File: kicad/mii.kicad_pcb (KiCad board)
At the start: 2 copper layers, 25.7 x 42.9 mm, 8 parts, among them IC1 RFM69, J1 Conn_Coaxial, J2 Conn_01x05, J3 Conn_01x03, J4 Conn_01x03, J5 Conn_01x03, J6 Conn_01x05, U1 WeMos_mini

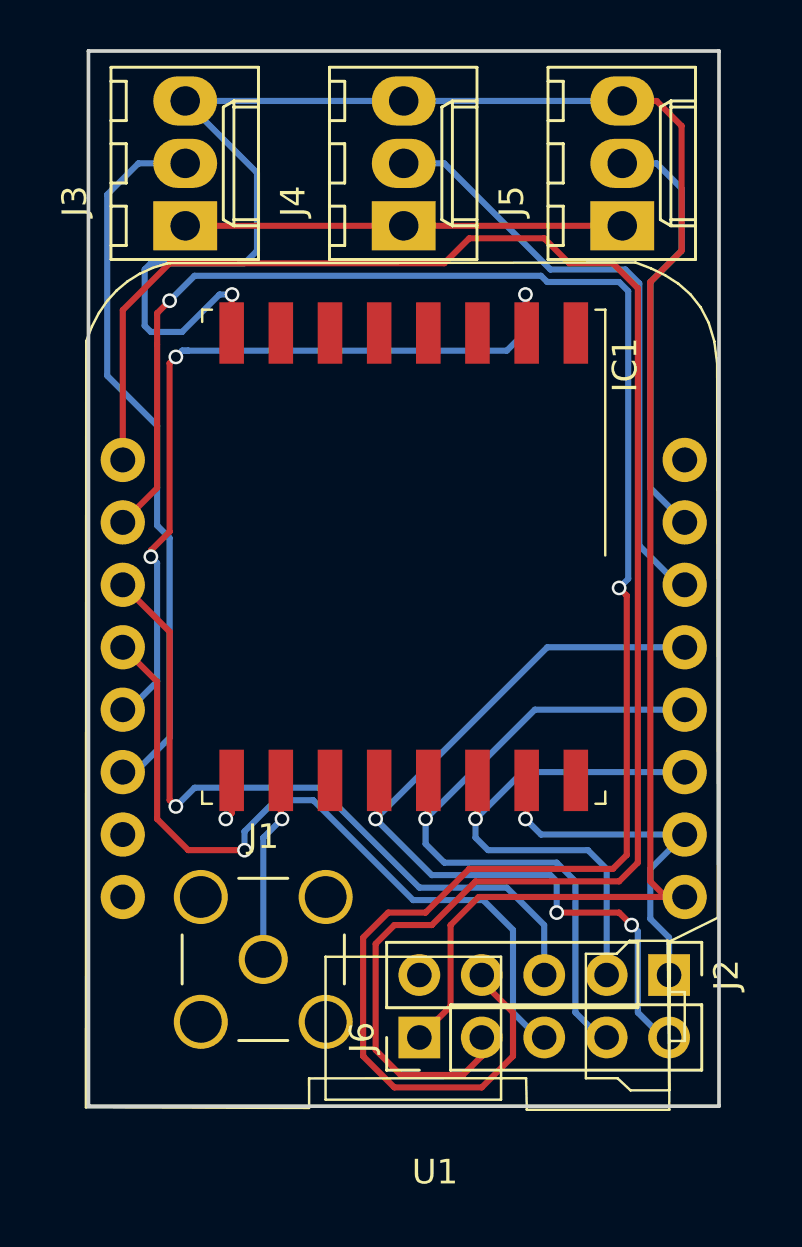
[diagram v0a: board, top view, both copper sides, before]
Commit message: Fix boundaries
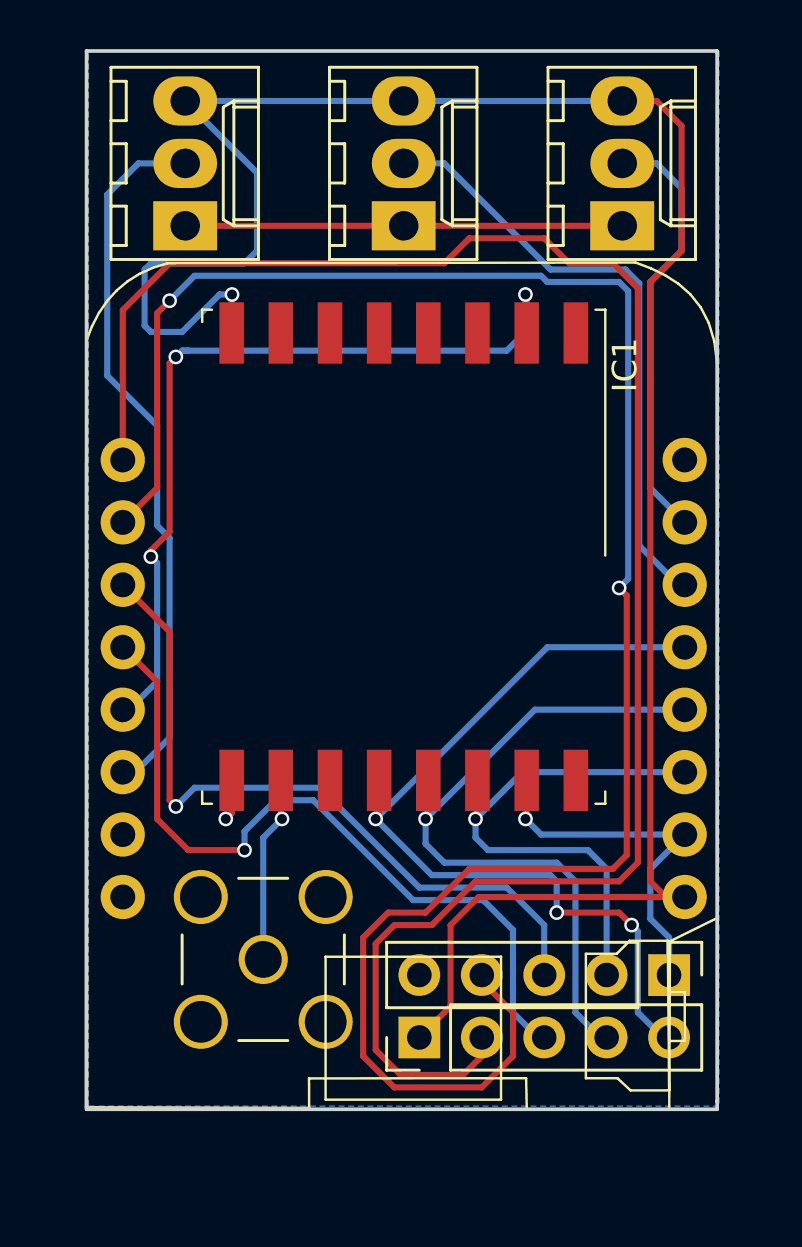
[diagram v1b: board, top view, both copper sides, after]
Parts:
- J1: value Conn_Coaxial -> Coaxial
- J2: value Conn_01x05 -> 3.3 TX SCL MISO SCK
- J3: value Conn_01x03 -> GND D4 3.3
- J4: value Conn_01x03 -> GND D0 3.3
- J5: value Conn_01x03 -> GND A0 3.3
- J6: value Conn_01x05 -> GND RX SDA MOSI NSS
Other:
- board size 25.7 x 42.9 mm -> 25.7 x 43.1 mm
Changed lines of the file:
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@@
     (area 106.92 82.88238 135.75 129.74)
     (thickness 1.6)
-    (drawings 4)
+    (drawings 6)
     (tracks 195)
     (zones 0)
@@
     (descr "Through hole straight pin header, 1x05, 2.54mm pitch, single row")
     (tags "Through hole pin header THT 1x05 2.54mm single row")
-    (fp_text reference J6 (at 0 -2.33 90) (layer F.SilkS)
-      (effects (font (size 1 1) (thickness 0.15)))
-    )
-    (fp_text value Conn_01x05 (at 0 12.49 90) (layer F.Fab)
-      (effects (font (size 1 1) (thickness 0.15)))
+    (fp_text reference J6 (at 0 -2.33 90) (layer F.SilkS) hide
+      (effects (font (size 1 1) (thickness 0.15)))
+    )
+    (fp_text value "GND RX SDA MOSI NSS" (at 4.318 5.08 180) (layer F.Fab)
+      (effects (font (size 0.7 0.7) (thickness 0.15)))
     )
     (fp_line (start -0.635 -1.27) (end 1.27 -1.27) (layer F.Fab) (width 0.1))
@@
   (module wemos_d1_mini:D1_mini_board (layer F.Cu)
     (at 121.285 109.855)
-    (fp_text reference U1 (at 1.27 18.81) (layer F.SilkS)
-      (effects (font (size 1 1) (thickness 0.15)))
-    )
-    (fp_text value WeMos_mini (at 1.27 -19.05) (layer F.Fab)
+    (fp_text reference U1 (at 1.27 18.81) (layer F.SilkS) hide
+      (effects (font (size 1 1) (thickness 0.15)))
+    )
+    (fp_text value WeMos_mini (at 1.27 -19.05) (layer F.Fab) hide
       (effects (font (size 1 1) (thickness 0.15)))
     )
@@
     (descr "Connector Headers with Friction Lock, 22-27-2031, http://www.molex.com/pdm_docs/sd/022272021_sd.pdf")
     (tags "connector molex kk_6410 22-27-2031")
-    (fp_text reference J3 (at 1 -4.5 90) (layer F.SilkS)
-      (effects (font (size 1 1) (thickness 0.15)))
-    )
-    (fp_text value Conn_01x03 (at 2.54 4.5 90) (layer F.Fab)
-      (effects (font (size 1 1) (thickness 0.15)))
+    (fp_text reference J3 (at 1 -4.5 90) (layer F.SilkS) hide
+      (effects (font (size 1 1) (thickness 0.15)))
+    )
+    (fp_text value "GND  D4 3.3" (at 2.286 -1.905 90) (layer F.Fab)
+      (effects (font (size 0.7 0.7) (thickness 0.15)))
     )
     (fp_line (start -1.47 -3.12) (end -1.47 3.08) (layer F.Fab) (width 0.12))
@@
     (fp_line (start 7 -3.55) (end 7 3.5) (layer F.CrtYd) (width 0.05))
     (fp_line (start 7 3.5) (end -1.9 3.5) (layer F.CrtYd) (width 0.05))
-    (fp_text user %R (at 2.54 0 90) (layer F.Fab)
+    (fp_text user %R (at 5.588 2.413 90) (layer F.Fab)
       (effects (font (size 1 1) (thickness 0.15)))
     )
@@
     (descr "SMA pcb through hole jack")
     (tags "SMA THT Jack Straight")
-    (fp_text reference J1 (at 0 -5) (layer F.SilkS)
-      (effects (font (size 1 1) (thickness 0.15)))
-    )
-    (fp_text value Conn_Coaxial (at 0 5) (layer F.Fab)
+    (fp_text reference J1 (at 0 -5) (layer F.SilkS) hide
+      (effects (font (size 1 1) (thickness 0.15)))
+    )
+    (fp_text value Coaxial (at 0 5) (layer F.Fab)
       (effects (font (size 1 1) (thickness 0.15)))
     )
@@
     (fp_line (start -1 -3.3) (end 1 -3.3) (layer F.SilkS) (width 0.12))
     (fp_line (start -1 3.3) (end 1 3.3) (layer F.SilkS) (width 0.12))
-    (fp_text user %R (at 0 -5) (layer F.Fab)
+    (fp_text user %R (at 2.286 -4.953) (layer F.Fab)
       (effects (font (size 1 1) (thickness 0.15)))
     )
@@
     (descr "Connector Headers with Friction Lock, 22-27-2031, http://www.molex.com/pdm_docs/sd/022272021_sd.pdf")
     (tags "connector molex kk_6410 22-27-2031")
-    (fp_text reference J4 (at 1 -4.5 90) (layer F.SilkS)
-      (effects (font (size 1 1) (thickness 0.15)))
-    )
-    (fp_text value Conn_01x03 (at 2.54 4.5 90) (layer F.Fab)
-      (effects (font (size 1 1) (thickness 0.15)))
+    (fp_text reference J4 (at 1 -4.5 90) (layer F.SilkS) hide
+      (effects (font (size 1 1) (thickness 0.15)))
+    )
+    (fp_text value "GND  D0 3.3" (at 2.286 -1.905 90) (layer F.Fab)
+      (effects (font (size 0.7 0.7) (thickness 0.15)))
     )
     (fp_line (start -1.47 -3.12) (end -1.47 3.08) (layer F.Fab) (width 0.12))
@@
     (fp_line (start 7 -3.55) (end 7 3.5) (layer F.CrtYd) (width 0.05))
     (fp_line (start 7 3.5) (end -1.9 3.5) (layer F.CrtYd) (width 0.05))
-    (fp_text user %R (at 2.54 0 90) (layer F.Fab)
+    (fp_text user %R (at 5.588 2.413 90) (layer F.Fab)
       (effects (font (size 1 1) (thickness 0.15)))
     )
@@
     (descr "Connector Headers with Friction Lock, 22-27-2031, http://www.molex.com/pdm_docs/sd/022272021_sd.pdf")
     (tags "connector molex kk_6410 22-27-2031")
-    (fp_text reference J5 (at 1 -4.5 90) (layer F.SilkS)
-      (effects (font (size 1 1) (thickness 0.15)))
-    )
-    (fp_text value Conn_01x03 (at 2.54 4.5 90) (layer F.Fab)
-      (effects (font (size 1 1) (thickness 0.15)))
+    (fp_text reference J5 (at 1 -4.5 90) (layer F.SilkS) hide
+      (effects (font (size 1 1) (thickness 0.15)))
+    )
+    (fp_text value "GND  A0 3.3" (at 2.286 -1.905 90) (layer F.Fab)
+      (effects (font (size 0.7 0.7) (thickness 0.15)))
     )
     (fp_line (start -1.47 -3.12) (end -1.47 3.08) (layer F.Fab) (width 0.12))
@@
     (fp_line (start 7 -3.55) (end 7 3.5) (layer F.CrtYd) (width 0.05))
     (fp_line (start 7 3.5) (end -1.9 3.5) (layer F.CrtYd) (width 0.05))
-    (fp_text user %R (at 2.54 0 90) (layer F.Fab)
+    (fp_text user %R (at 5.588 2.413 90) (layer F.Fab)
       (effects (font (size 1 1) (thickness 0.15)))
     )
@@
     (descr "Through hole straight pin header, 1x05, 2.54mm pitch, single row")
     (tags "Through hole pin header THT 1x05 2.54mm single row")
-    (fp_text reference J2 (at 0 -2.33 270) (layer F.SilkS)
-      (effects (font (size 1 1) (thickness 0.15)))
-    )
-    (fp_text value Conn_01x05 (at 0 12.49 270) (layer F.Fab)
-      (effects (font (size 1 1) (thickness 0.15)))
+    (fp_text reference J2 (at 0 -2.33 270) (layer F.SilkS) hide
+      (effects (font (size 1 1) (thickness 0.15)))
+    )
+    (fp_text value "3.3  TX  SCL MISO SCK" (at 4.318 4.826 360) (layer F.Fab)
+      (effects (font (size 0.7 0.7) (thickness 0.15)))
     )
     (fp_line (start -0.635 -1.27) (end 1.27 -1.27) (layer F.Fab) (width 0.1))
@@
     (fp_line (start 1.8 11.95) (end 1.8 -1.8) (layer F.CrtYd) (width 0.05))
     (fp_line (start 1.8 -1.8) (end -1.8 -1.8) (layer F.CrtYd) (width 0.05))
-    (fp_text user %R (at 0 5.08 360) (layer F.Fab)
+    (fp_text user %R (at -0.508 11.938 360) (layer F.Fab)
       (effects (font (size 1 1) (thickness 0.15)))
     )
@@
     )
   )
-  (gr_line (start 134.112 125.984) (end 134.112 83.058) (angle 90) (layer Edge.Cuts) (width 0.15))
-  (gr_line (start 108.458 125.984) (end 108.458 83.058) (angle 90) (layer Edge.Cuts) (width 0.15))
-  (gr_line (start 108.458 125.984) (end 134.112 125.984) (angle 90) (layer Edge.Cuts) (width 0.15))
-  (gr_line (start 108.458 83.058) (end 134.112 83.058) (angle 90) (layer Edge.Cuts) (width 0.15))
+  (gr_line (start 108.3818 126.111) (end 108.3818 83.058) (angle 90) (layer Edge.Cuts) (width 0.15))
+  (gr_line (start 134.0358 126.111) (end 108.3818 126.111) (angle 90) (layer Edge.Cuts) (width 0.15))
+  (gr_line (start 134.0358 125.7808) (end 134.0358 126.111) (angle 90) (layer Edge.Cuts) (width 0.15))
+  (gr_line (start 134.0358 125.7808) (end 134.0358 83.058) (angle 90) (layer Edge.Cuts) (width 0.15))
+  (gr_line (start 134.0104 83.058) (end 134.0104 83.0834) (angle 90) (layer Edge.Cuts) (width 0.15))
+  (gr_line (start 108.3818 83.058) (end 134.0104 83.058) (angle 90) (layer Edge.Cuts) (width 0.15))
   (segment (start 132.08 120.65) (end 132.08 119.126) (width 0.25) (layer B.Cu) (net 10) (status 10))
   (segment (start 131.318 116.332) (end 132.715 114.935) (width 0.25) (layer B.Cu) (net 10) (status 20))
